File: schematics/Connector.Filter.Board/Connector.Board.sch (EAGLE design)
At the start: 220 parts, among them U1 AD8244, U10 AD8244, U11 AD8244, U12 AD8244, U13 AD8244, U14 AD8244, U15 AD8244, U16 AD8244, U17 AD8244, U18 AD8244, U19 AD8244, U2 AD8244, U20 AD8244, U21 AD8244, U22 AD8244, U23 AD8244, U24 AD8244, U3 AD8244, U4 AD8244, U5 AD8244, U6 AD8244, U7 AD8244, U8 AD8244, U9 AD8244, X1 EEGCON, X2 EITCON

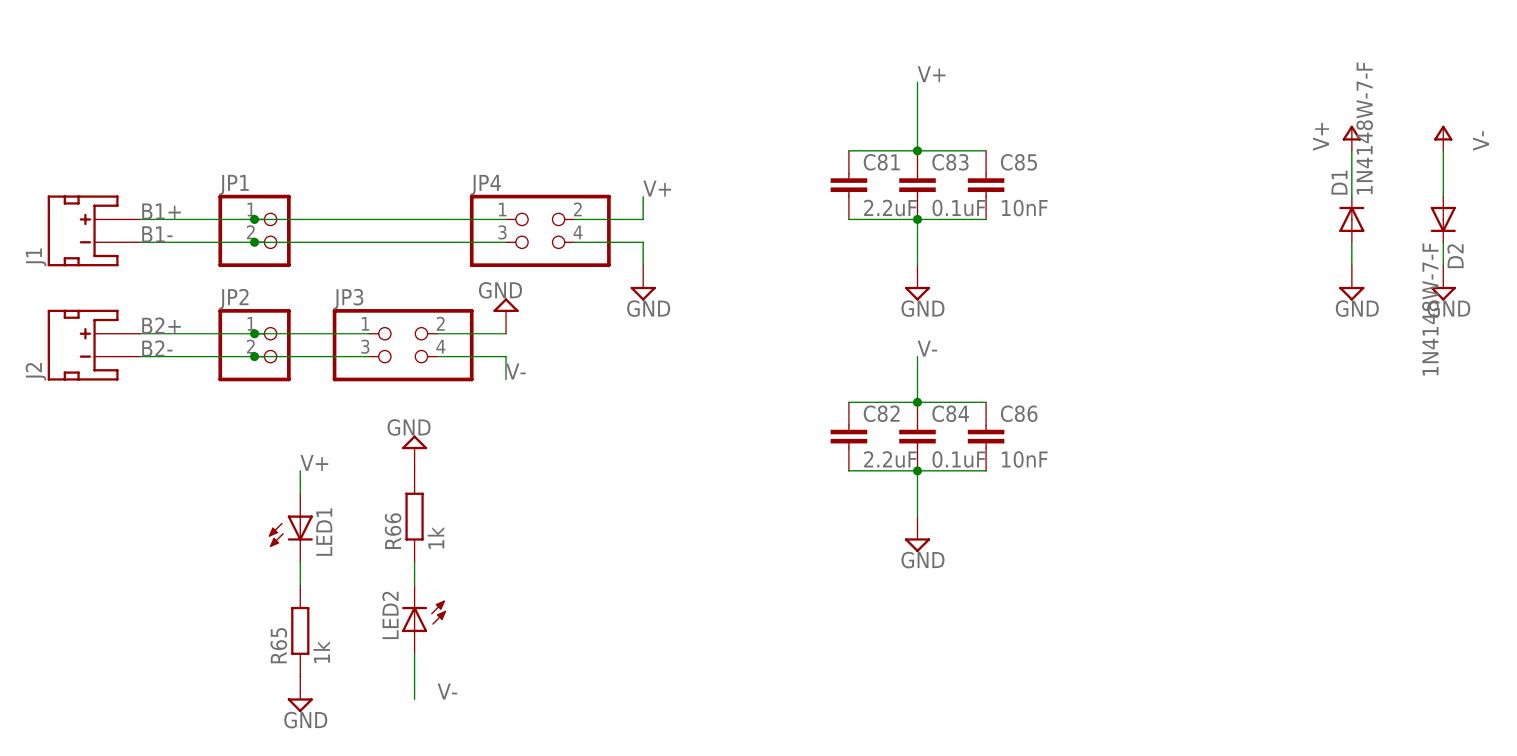
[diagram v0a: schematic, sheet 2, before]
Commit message: Finished Board
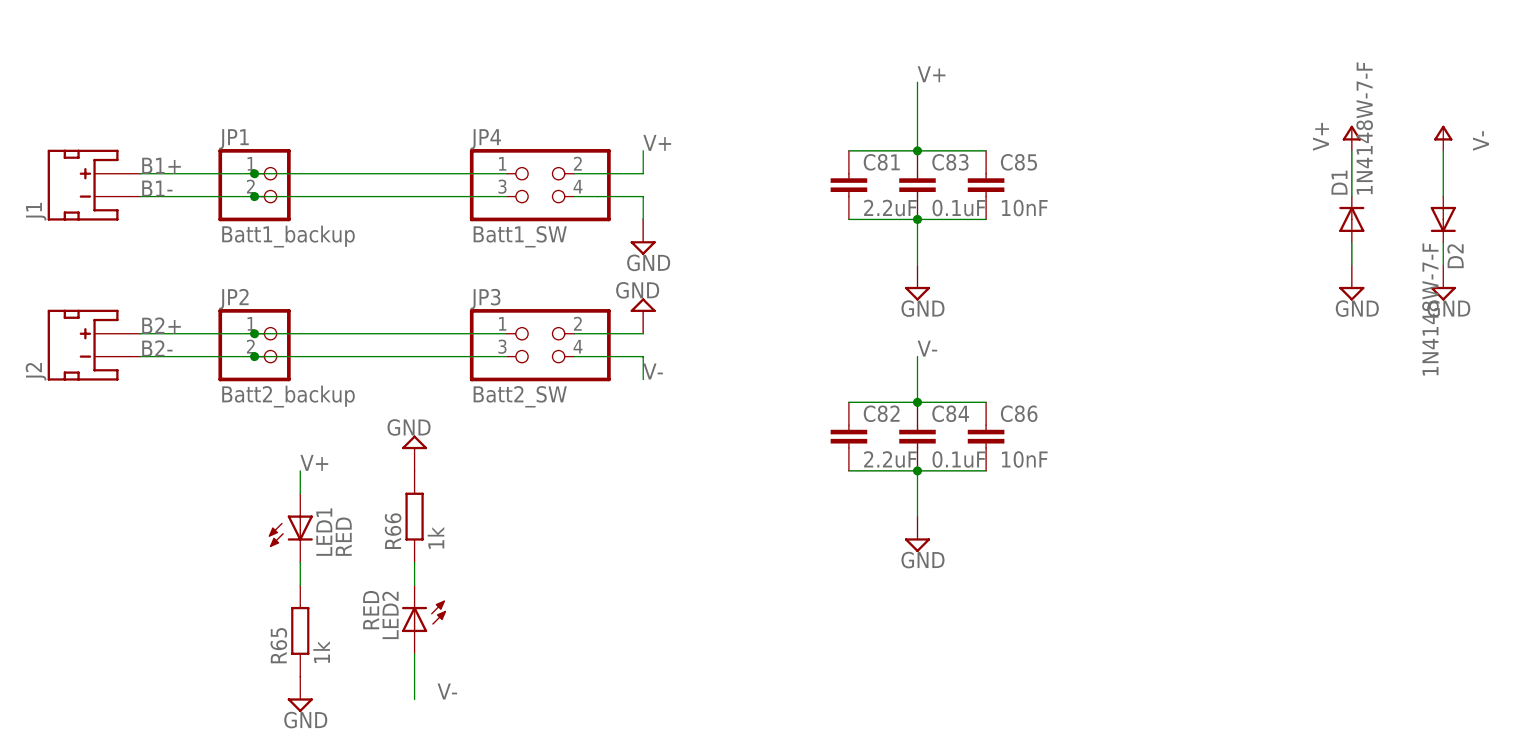
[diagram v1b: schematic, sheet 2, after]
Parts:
- J1: value (none) -> V+BATT
- J2: value (none) -> V-BATT
- JP1: value (none) -> Batt1_backup
- JP2: value (none) -> Batt2_backup
- JP3: value (none) -> Batt2_SW
- JP4: value (none) -> Batt1_SW
- LED1, LED2: value (none) -> RED
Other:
- moved on the sheet: J1, JP1, JP3, JP4
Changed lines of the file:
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@@
 <layer number="20" name="Dimension" color="15" fill="1" visible="yes" active="no"/>
 <layer number="21" name="tPlace" color="7" fill="1" visible="yes" active="no"/>
-<layer number="22" name="bPlace" color="7" fill="1" visible="yes" active="no"/>
+<layer number="22" name="bPlace" color="14" fill="1" visible="yes" active="no"/>
 <layer number="23" name="tOrigins" color="15" fill="1" visible="yes" active="no"/>
 <layer number="24" name="bOrigins" color="15" fill="1" visible="yes" active="no"/>
 <layer number="25" name="tNames" color="7" fill="1" visible="yes" active="no"/>
-<layer number="26" name="bNames" color="7" fill="1" visible="yes" active="no"/>
+<layer number="26" name="bNames" color="14" fill="1" visible="yes" active="no"/>
 <layer number="27" name="tValues" color="7" fill="1" visible="yes" active="no"/>
 <layer number="28" name="bValues" color="7" fill="1" visible="yes" active="no"/>
@@
 <layer number="50" name="dxf" color="7" fill="1" visible="yes" active="no"/>
 <layer number="51" name="tDocu" color="7" fill="1" visible="yes" active="no"/>
-<layer number="52" name="bDocu" color="7" fill="1" visible="yes" active="no"/>
+<layer number="52" name="bDocu" color="14" fill="1" visible="yes" active="no"/>
 <layer number="53" name="tGND_GNDA" color="7" fill="9" visible="yes" active="no"/>
 <layer number="54" name="bGND_GNDA" color="1" fill="9" visible="yes" active="no"/>
@@
 <part name="TP31" library="connector_board_lib" deviceset="TOUCHPROOF" device=""/>
 <part name="TP32" library="connector_board_lib" deviceset="TOUCHPROOF" device=""/>
-<part name="JP1" library="pinhead" deviceset="PINHD-1X2" device=""/>
-<part name="JP2" library="pinhead" deviceset="PINHD-1X2" device=""/>
+<part name="JP1" library="pinhead" deviceset="PINHD-1X2" device="" value="Batt1_backup"/>
+<part name="JP2" library="pinhead" deviceset="PINHD-1X2" device="" value="Batt2_backup"/>
 <part name="SUPPLY3" library="supply2" deviceset="GND" device=""/>
 <part name="SUPPLY4" library="supply2" deviceset="GND" device=""/>
@@
 <part name="R24" library="resistor" deviceset="R-EU_" device="R0402" value="1M"/>
 <part name="GND24" library="supply1" deviceset="GND" device=""/>
-<part name="J1" library="SparkFun-Connectors" deviceset="JST_2MM_MALE" device=""/>
-<part name="J2" library="SparkFun-Connectors" deviceset="JST_2MM_MALE" device=""/>
-<part name="JP4" library="pinhead" deviceset="PINHD-2X2" device=""/>
-<part name="JP3" library="pinhead" deviceset="PINHD-2X2" device=""/>
-<part name="LED1" library="led" deviceset="LED" device="SML0805"/>
-<part name="LED2" library="led" deviceset="LED" device="SML0805"/>
+<part name="J1" library="SparkFun-Connectors" deviceset="JST_2MM_MALE" device="" value="V+BATT"/>
+<part name="J2" library="SparkFun-Connectors" deviceset="JST_2MM_MALE" device="" value="V-BATT"/>
+<part name="JP4" library="pinhead" deviceset="PINHD-2X2" device="" value="Batt1_SW"/>
+<part name="JP3" library="pinhead" deviceset="PINHD-2X2" device="" value="Batt2_SW"/>
+<part name="LED1" library="led" deviceset="LED" device="SML0805" value="RED"/>
+<part name="LED2" library="led" deviceset="LED" device="SML0805" value="RED"/>
 <part name="R65" library="resistor" deviceset="R-EU_" device="R0402" value="1k"/>
 <part name="SUPPLY1" library="supply2" deviceset="GND" device=""/>
@@
 </plain>
 <instances>
-<instance part="JP1" gate="G$1" x="-101.6" y="109.22"/>
+<instance part="JP1" gate="G$1" x="-101.6" y="114.3"/>
 <instance part="JP2" gate="G$1" x="-101.6" y="96.52"/>
-<instance part="SUPPLY3" gate="GND" x="-76.2" y="101.6" rot="R180"/>
-<instance part="SUPPLY4" gate="GND" x="-60.96" y="104.14"/>
+<instance part="SUPPLY3" gate="GND" x="-60.96" y="101.6" rot="R180"/>
+<instance part="SUPPLY4" gate="GND" x="-60.96" y="109.22"/>
 <instance part="C83" gate="G$1" x="-30.48" y="116.84"/>
 <instance part="C84" gate="G$1" x="-30.48" y="88.9"/>
@@
 <instance part="C82" gate="G$1" x="-38.1" y="88.9"/>
 <instance part="C86" gate="G$1" x="-22.86" y="88.9"/>
-<instance part="J1" gate="G$1" x="-121.92" y="109.22" rot="R90"/>
+<instance part="J1" gate="G$1" x="-121.92" y="114.3" rot="R90"/>
 <instance part="J2" gate="G$1" x="-121.92" y="96.52" rot="R90"/>
-<instance part="JP4" gate="A" x="-71.12" y="109.22"/>
-<instance part="JP3" gate="A" x="-86.36" y="96.52"/>
+<instance part="JP4" gate="A" x="-71.12" y="114.3"/>
+<instance part="JP3" gate="A" x="-71.12" y="96.52"/>
 <instance part="LED1" gate="G$1" x="-99.06" y="78.74"/>
 <instance part="LED2" gate="G$1" x="-86.36" y="66.04" rot="R180"/>
@@
 <net name="V-" class="0">
 <segment>
-<wire x1="-76.2" y1="96.52" x2="-76.2" y2="93.98" width="0.1524" layer="91"/>
-<label x="-76.2" y="93.98" size="1.778" layer="95"/>
+<wire x1="-60.96" y1="96.52" x2="-60.96" y2="93.98" width="0.1524" layer="91"/>
+<label x="-60.96" y="93.98" size="1.778" layer="95"/>
 <pinref part="JP3" gate="A" pin="4"/>
-<wire x1="-83.82" y1="96.52" x2="-76.2" y2="96.52" width="0.1524" layer="91"/>
+<wire x1="-68.58" y1="96.52" x2="-60.96" y2="96.52" width="0.1524" layer="91"/>
 </segment>
 <segment>
@@
 <net name="V+" class="0">
 <segment>
-<wire x1="-60.96" y1="111.76" x2="-60.96" y2="114.3" width="0.1524" layer="91"/>
-<label x="-60.96" y="114.3" size="1.778" layer="95"/>
+<wire x1="-60.96" y1="116.84" x2="-60.96" y2="119.38" width="0.1524" layer="91"/>
+<label x="-60.96" y="119.38" size="1.778" layer="95"/>
 <pinref part="JP4" gate="A" pin="2"/>
-<wire x1="-68.58" y1="111.76" x2="-60.96" y2="111.76" width="0.1524" layer="91"/>
+<wire x1="-68.58" y1="116.84" x2="-60.96" y2="116.84" width="0.1524" layer="91"/>
 </segment>
 <segment>
@@
 </segment>
 <segment>
-<wire x1="-66.04" y1="109.22" x2="-60.96" y2="109.22" width="0.1524" layer="91"/>
+<wire x1="-66.04" y1="114.3" x2="-60.96" y2="114.3" width="0.1524" layer="91"/>
 <pinref part="SUPPLY4" gate="GND" pin="GND"/>
-<wire x1="-60.96" y1="109.22" x2="-60.96" y2="106.68" width="0.1524" layer="91"/>
+<wire x1="-60.96" y1="114.3" x2="-60.96" y2="111.76" width="0.1524" layer="91"/>
 <pinref part="JP4" gate="A" pin="4"/>
-<wire x1="-66.04" y1="109.22" x2="-68.58" y2="109.22" width="0.1524" layer="91"/>
+<wire x1="-66.04" y1="114.3" x2="-68.58" y2="114.3" width="0.1524" layer="91"/>
 </segment>
 <segment>
 <pinref part="JP3" gate="A" pin="2"/>
 <pinref part="SUPPLY3" gate="GND" pin="GND"/>
-<wire x1="-83.82" y1="99.06" x2="-76.2" y2="99.06" width="0.1524" layer="91"/>
+<wire x1="-68.58" y1="99.06" x2="-60.96" y2="99.06" width="0.1524" layer="91"/>
 </segment>
 <segment>
@@
 <pinref part="J1" gate="G$1" pin="+"/>
 <pinref part="JP1" gate="G$1" pin="1"/>
-<wire x1="-116.84" y1="111.76" x2="-104.14" y2="111.76" width="0.1524" layer="91"/>
-<label x="-116.84" y="111.76" size="1.778" layer="95"/>
+<wire x1="-116.84" y1="116.84" x2="-104.14" y2="116.84" width="0.1524" layer="91"/>
+<label x="-116.84" y="116.84" size="1.778" layer="95"/>
 <pinref part="JP4" gate="A" pin="1"/>
-<wire x1="-104.14" y1="111.76" x2="-76.2" y2="111.76" width="0.1524" layer="91"/>
-<junction x="-104.14" y="111.76"/>
+<wire x1="-104.14" y1="116.84" x2="-76.2" y2="116.84" width="0.1524" layer="91"/>
+<junction x="-104.14" y="116.84"/>
 </segment>
 </net>
@@
 <pinref part="J1" gate="G$1" pin="-"/>
 <pinref part="JP1" gate="G$1" pin="2"/>
-<wire x1="-116.84" y1="109.22" x2="-104.14" y2="109.22" width="0.1524" layer="91"/>
-<label x="-116.84" y="109.22" size="1.778" layer="95"/>
+<wire x1="-116.84" y1="114.3" x2="-104.14" y2="114.3" width="0.1524" layer="91"/>
+<label x="-116.84" y="114.3" size="1.778" layer="95"/>
 <pinref part="JP4" gate="A" pin="3"/>
-<wire x1="-104.14" y1="109.22" x2="-76.2" y2="109.22" width="0.1524" layer="91"/>
-<junction x="-104.14" y="109.22"/>
+<wire x1="-104.14" y1="114.3" x2="-76.2" y2="114.3" width="0.1524" layer="91"/>
+<junction x="-104.14" y="114.3"/>
 </segment>
 </net>
@@
 <label x="-116.84" y="99.06" size="1.778" layer="95"/>
 <pinref part="JP3" gate="A" pin="1"/>
-<wire x1="-104.14" y1="99.06" x2="-91.44" y2="99.06" width="0.1524" layer="91"/>
+<wire x1="-104.14" y1="99.06" x2="-76.2" y2="99.06" width="0.1524" layer="91"/>
 <junction x="-104.14" y="99.06"/>
 </segment>
@@
 <label x="-116.84" y="96.52" size="1.778" layer="95"/>
 <pinref part="JP3" gate="A" pin="3"/>
-<wire x1="-104.14" y1="96.52" x2="-91.44" y2="96.52" width="0.1524" layer="91"/>
+<wire x1="-104.14" y1="96.52" x2="-76.2" y2="96.52" width="0.1524" layer="91"/>
 <junction x="-104.14" y="96.52"/>
 </segment>
